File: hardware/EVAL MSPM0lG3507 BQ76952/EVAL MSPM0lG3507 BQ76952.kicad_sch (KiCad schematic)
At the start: 68 parts, among them J1 Conn_01x09_Socket, J10 Screw_Terminal_01x02, J11 Screw_Terminal_01x02, J12 Screw_Terminal_01x02, J13 Screw_Terminal_01x02, J14 Screw_Terminal_01x02, J17 Conn_02x02_Odd_Even, J2 Conn_02x05_Odd_Even, J3 Conn_01x04_Pin, J4 Screw_Terminal_01x02, J5 Conn_01x09_Socket, J6 Conn_01x02_Pin, J7 Screw_Terminal_01x02, J8 Screw_Terminal_01x02, J9 Screw_Terminal_01x02, Q6 2N7002, SW1 SW_Push, SW2 SW_Push, U2 MCU-MSM0G3507SPM, U6 TPD4E05U06DQA, U7 TPD4E05U06DQA

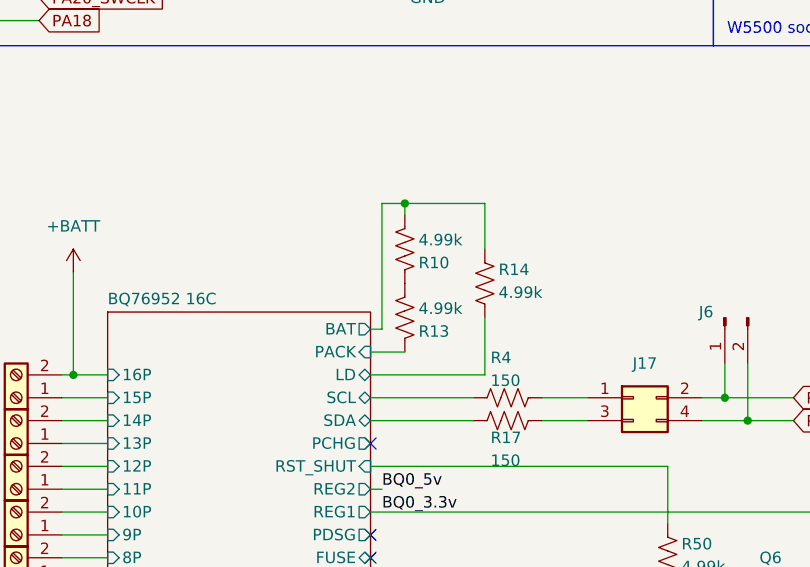
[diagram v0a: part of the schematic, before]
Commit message: sGDdfsddsf
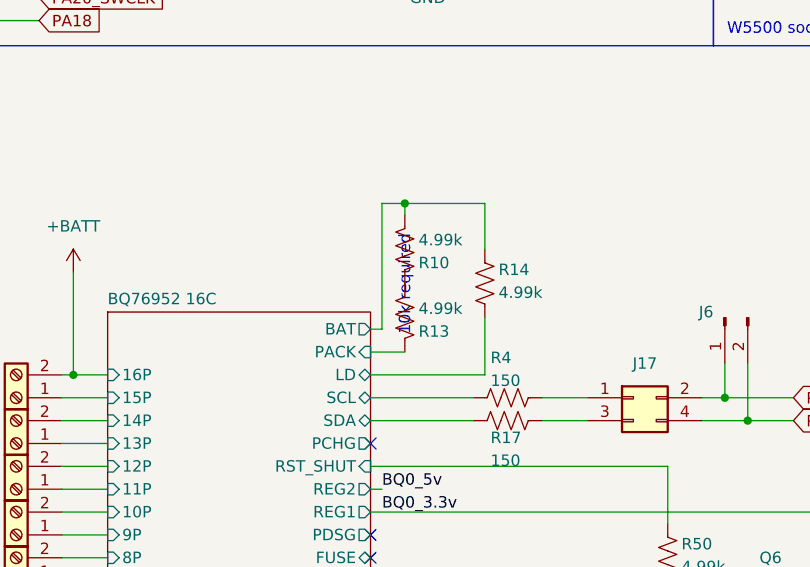
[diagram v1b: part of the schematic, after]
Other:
- note added: "10k required"
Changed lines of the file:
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@@
+		)
+	)
+	(text "10k required"
+		(exclude_from_sim no)
+		(at 87.63 123.444 90)
+		(effects
+			(font
+				(size 1.27 1.27)
+			)
 		)
 	)
